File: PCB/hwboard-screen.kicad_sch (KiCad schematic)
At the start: 1 part, among them J1 Conn_01x40

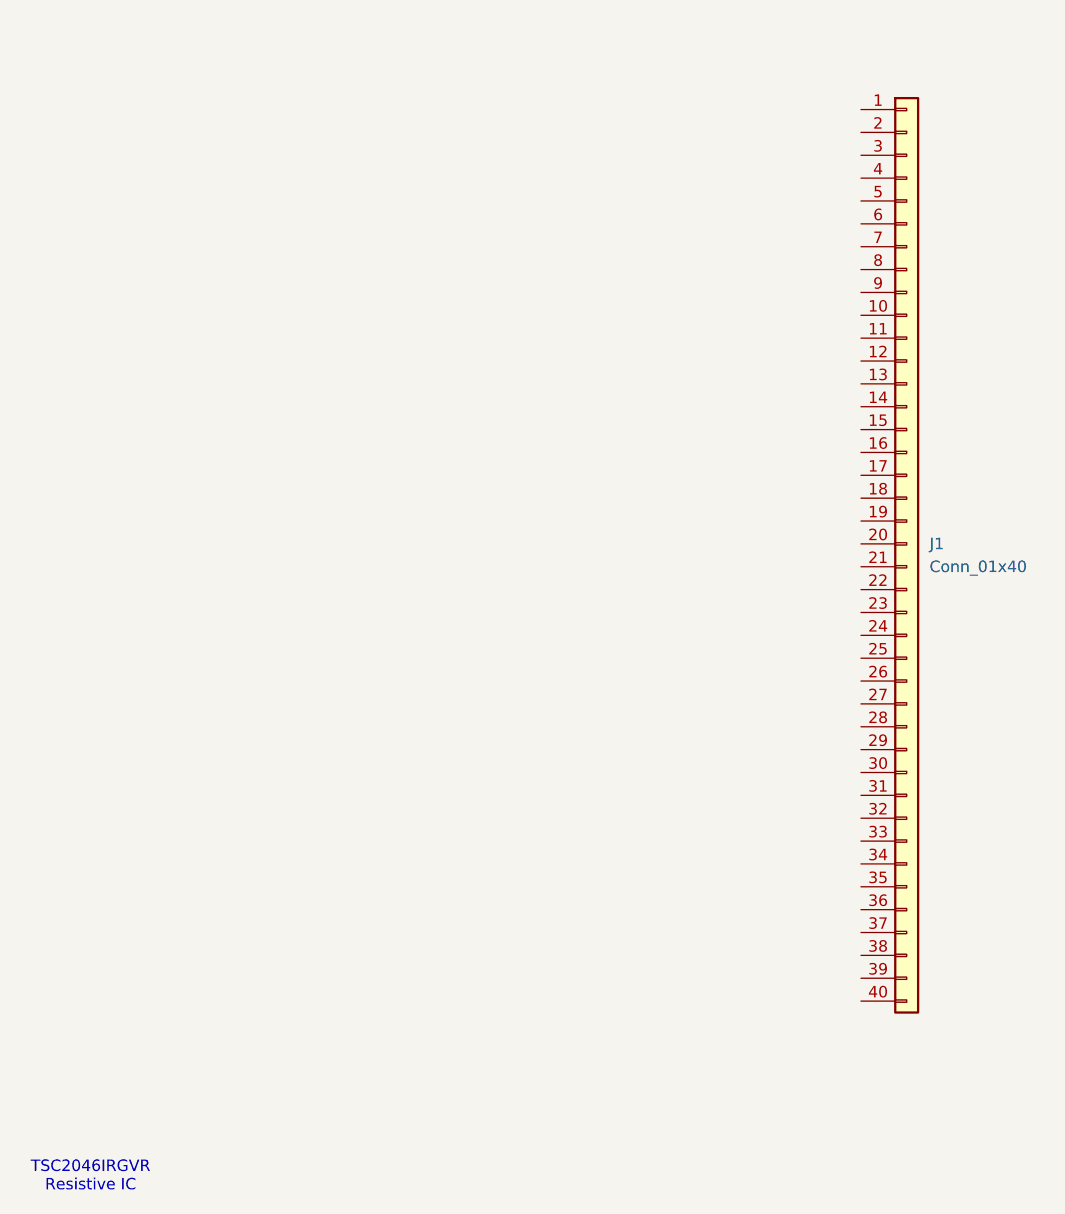
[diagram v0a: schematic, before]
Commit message: add maybe layout and pcb for screen
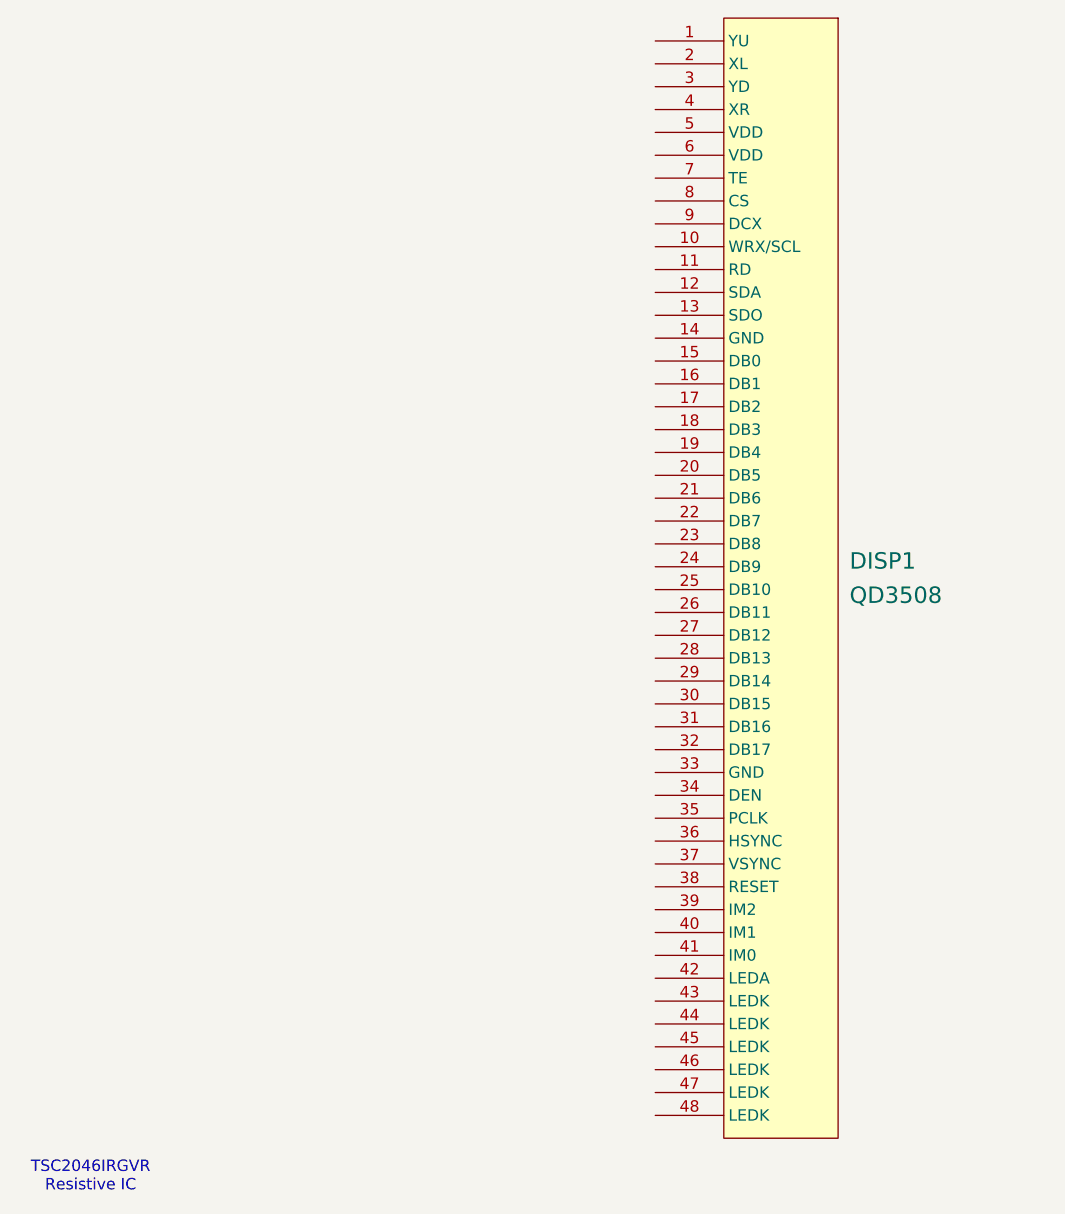
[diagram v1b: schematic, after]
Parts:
- removed J1: Conn_01x40, symbol Connector_Generic:Conn_01x40
- added DISP1: QD3508, G__project_3.5inch_3.5inch_common_spi_ctp_PCB_3.5inch_Common_SPI_CTP.PcbLib:3.5-QD3503, symbol hwboard-bike-computer:QD3508
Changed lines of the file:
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@@
 	)
 	(symbol
-		(lib_id "Connector_Generic:Conn_01x40")
-		(at 201.93 88.9 0)
+		(lib_id "hwboard-bike-computer:QD3508")
+		(at 173.99 30.48 0)
 		(unit 1)
 		(exclude_from_sim no)
@@
 		(dnp no)
 		(fields_autoplaced yes)
-		(property "Reference" "J1"
-			(at 204.47 88.8999 0)
+		(property "Reference" "DISP1"
+			(at 195.58 90.8049 0)
 			(effects
 				(font
-					(size 1.27 1.27)
+					(size 1.8288 1.8288)
 				)
 				(justify left)
 			)
 		)
-		(property "Value" "Conn_01x40"
-			(at 204.47 91.4399 0)
+		(property "Value" "QD3508"
+			(at 195.58 94.6149 0)
 			(effects
 				(font
-					(size 1.27 1.27)
+					(size 1.8288 1.8288)
 				)
 				(justify left)
 			)
 		)
-		(property "Footprint" ""
-			(at 201.93 88.9 0)
+		(property "Footprint" "G__project_3.5inch_3.5inch_common_spi_ctp_PCB_3.5inch_Common_SPI_CTP.PcbLib:3.5-QD3503"
+			(at 173.99 30.48 0)
 			(effects
 				(font
@@
 			)
 		)
-		(property "Datasheet" "~"
-			(at 201.93 88.9 0)
+		(property "Datasheet" ""
+			(at 173.99 30.48 0)
 			(effects
 				(font
@@
 			)
 		)
-		(property "Description" "Generic connector, single row, 01x40, script generated (kicad-library-utils/schlib/autogen/connector/)"
-			(at 201.93 88.9 0)
+		(property "Description" ""
+			(at 173.99 30.48 0)
 			(effects
 				(font
@@
 			)
 		)
-		(pin "31"
-		)
 		(pin "38"
-		)
-		(pin "8"
-		)
-		(pin "20"
-		)
-		(pin "18"
-		)
-		(pin "11"
-		)
-		(pin "34"
-		)
-		(pin "23"
-		)
-		(pin "39"
-		)
-		(pin "35"
-		)
-		(pin "27"
-		)
-		(pin "36"
-		)
-		(pin "28"
 		)
 		(pin "29"
 		)
-		(pin "24"
-		)
-		(pin "12"
-		)
-		(pin "25"
-		)
-		(pin "26"
-		)
-		(pin "37"
-		)
-		(pin "9"
-		)
-		(pin "13"
-		)
-		(pin "3"
-		)
-		(pin "1"
+		(pin "22"
 		)
 		(pin "4"
-		)
-		(pin "2"
-		)
-		(pin "5"
-		)
-		(pin "10"
-		)
-		(pin "17"
-		)
-		(pin "14"
-		)
-		(pin "40"
-		)
-		(pin "30"
-		)
-		(pin "33"
-		)
-		(pin "19"
-		)
-		(pin "22"
 		)
 		(pin "7"
@@
 		(pin "6"
 		)
-		(pin "16"
+		(pin "5"
+		)
+		(pin "2"
+		)
+		(pin "1"
+		)
+		(pin "19"
+		)
+		(pin "17"
+		)
+		(pin "39"
 		)
 		(pin "21"
 		)
+		(pin "35"
+		)
+		(pin "18"
+		)
+		(pin "8"
+		)
+		(pin "15"
+		)
+		(pin "16"
+		)
+		(pin "43"
+		)
+		(pin "44"
+		)
+		(pin "34"
+		)
+		(pin "10"
+		)
+		(pin "33"
+		)
+		(pin "36"
+		)
+		(pin "40"
+		)
+		(pin "28"
+		)
+		(pin "23"
+		)
+		(pin "42"
+		)
+		(pin "11"
+		)
+		(pin "45"
+		)
+		(pin "30"
+		)
+		(pin "27"
+		)
+		(pin "48"
+		)
+		(pin "37"
+		)
+		(pin "25"
+		)
+		(pin "24"
+		)
+		(pin "47"
+		)
+		(pin "26"
+		)
+		(pin "41"
+		)
+		(pin "9"
+		)
+		(pin "31"
+		)
 		(pin "32"
 		)
-		(pin "15"
+		(pin "12"
+		)
+		(pin "20"
+		)
+		(pin "14"
+		)
+		(pin "46"
+		)
+		(pin "3"
+		)
+		(pin "13"
 		)
 		(instances
 			(project ""
 				(path "/8c0f76b9-ee42-4bcf-bb95-09772e367402/4b830c8b-a993-4513-b498-b6b511f6381b"
-					(reference "J1")
+					(reference "DISP1")
 					(unit 1)
 				)
